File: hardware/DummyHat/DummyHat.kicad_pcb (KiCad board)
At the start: 2 copper layers, 1 part, among them U1 7404

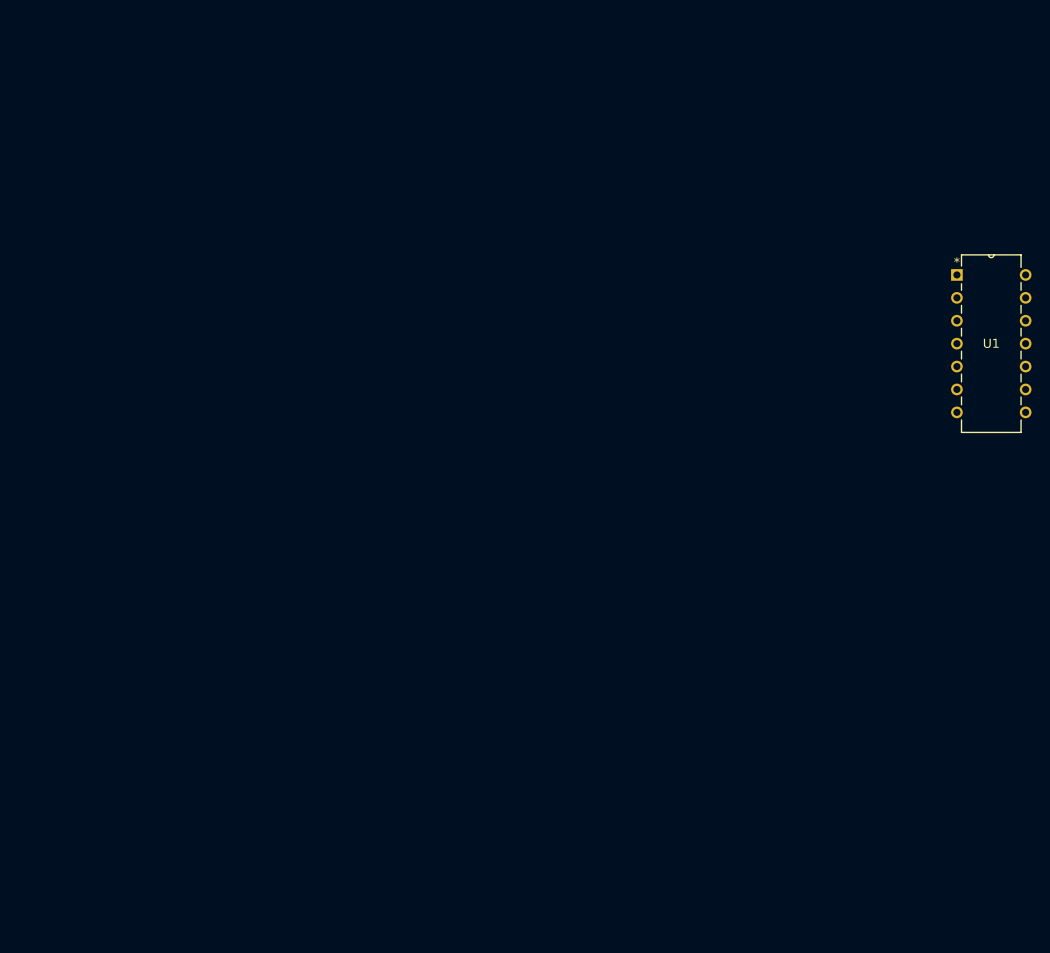
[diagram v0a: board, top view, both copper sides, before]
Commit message: Finish First Dummy Hat Design
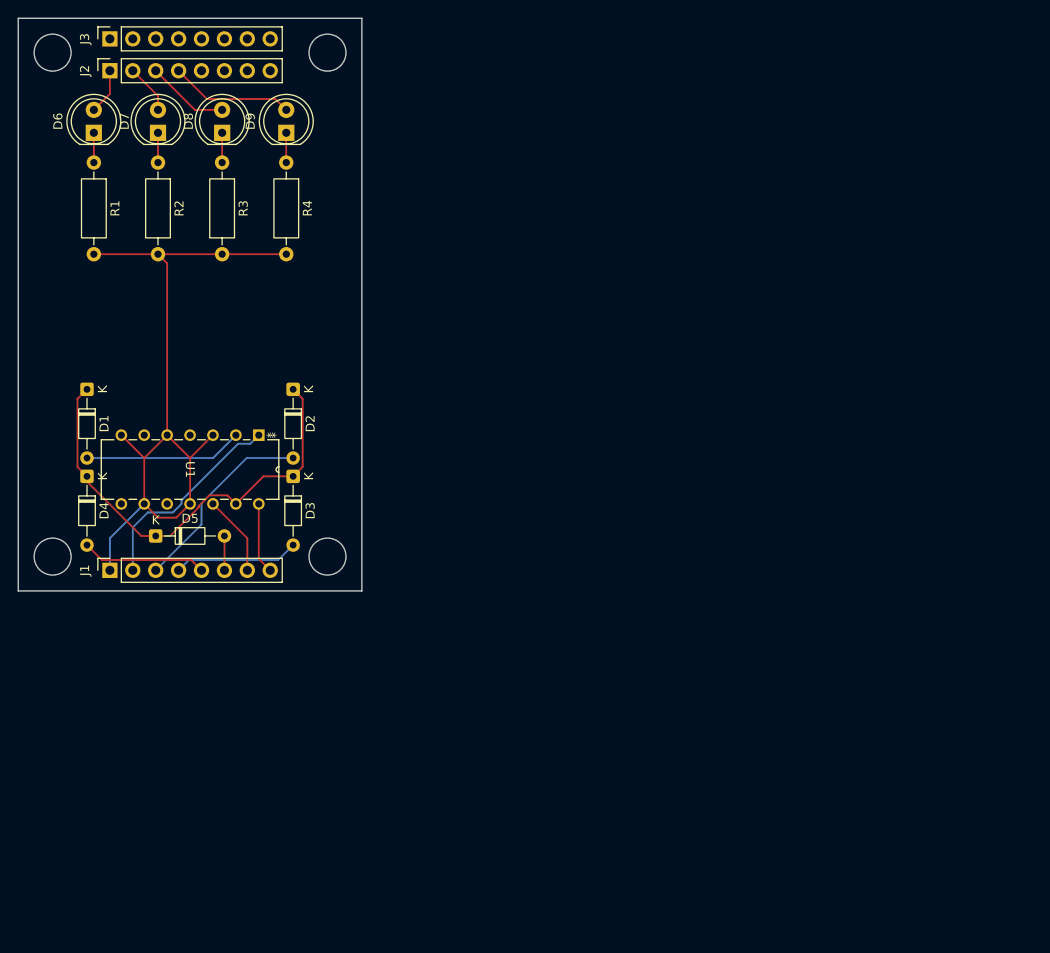
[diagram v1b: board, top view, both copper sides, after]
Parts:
- added D1: D, Diode_THT:D_DO-34_SOD68_P7.62mm_Horizontal, F.Cu at (58.4, 91.9)
- added D2: D, Diode_THT:D_DO-34_SOD68_P7.62mm_Horizontal, F.Cu at (81.3, 91.9)
- added D3: D, Diode_THT:D_DO-34_SOD68_P7.62mm_Horizontal, F.Cu at (81.3, 101.6)
- added D4: D, Diode_THT:D_DO-34_SOD68_P7.62mm_Horizontal, F.Cu at (58.4, 101.6)
- added D5: D, Diode_THT:D_DO-34_SOD68_P7.62mm_Horizontal, F.Cu at (66.0, 108.2)
- added D6: LED, LED_THT:LED_D5.0mm, F.Cu at (59.2, 63.5)
- added D7: LED, LED_THT:LED_D5.0mm, F.Cu at (66.3, 63.5)
- added D8: LED, LED_THT:LED_D5.0mm, F.Cu at (73.4, 63.5)
- added D9: LED, LED_THT:LED_D5.0mm, F.Cu at (80.5, 63.5)
- added J1: Conn_01x08_Socket, Connector_PinSocket_2.54mm:PinSocket_1x08_P2.54mm_Vertical, F.Cu at (61.0, 112.0)
- added J2: Conn_01x08_Socket, Connector_PinSocket_2.54mm:PinSocket_1x08_P2.54mm_Vertical, F.Cu at (61.0, 56.6)
- added J3: Conn_01x08_Socket, Connector_PinSocket_2.54mm:PinSocket_1x08_P2.54mm_Vertical, F.Cu at (61.0, 53.1)
- added R1: R, Resistor_THT:R_Axial_DIN0207_L6.3mm_D2.5mm_P10.16mm_Horizontal, F.Cu at (59.2, 66.8)
- added R2: R, Resistor_THT:R_Axial_DIN0207_L6.3mm_D2.5mm_P10.16mm_Horizontal, F.Cu at (66.3, 66.8)
- added R3: R, Resistor_THT:R_Axial_DIN0207_L6.3mm_D2.5mm_P10.16mm_Horizontal, F.Cu at (73.4, 66.8)
- added R4: R, Resistor_THT:R_Axial_DIN0207_L6.3mm_D2.5mm_P10.16mm_Horizontal, F.Cu at (80.5, 66.8)
- U1: value 7404 -> 74HC04
- moved U1 100.8 mm to (62.2, 104.6), turned to -90 degrees
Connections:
- U1 pad 1: unconnected-(U1-Pad1) -> I0
- U1 pad 11: unconnected-(U1-Pad11) -> GND
- U1 pad 12: unconnected-(U1-Pad12) -> RESP
- U1 pad 13: unconnected-(U1-Pad13) -> Net-(D1-K)
- U1 pad 2: unconnected-(U1-Pad2) -> Net-(D1-A)
- U1 pad 3: unconnected-(U1-Pad3) -> GND
- U1 pad 5: unconnected-(U1-Pad5) -> GND
- U1 pad 9: unconnected-(U1-Pad9) -> GND
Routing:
- net GND: track 0.00 -> 81.6 mm
- net Net-(D1-K): track 0.00 -> 50.6 mm
- net I0: track 0.00 -> 23.2 mm
- net I1: track 0.00 -> 21.8 mm
- net Net-(D1-A): track 0.00 -> 17.6 mm
- net I2: track 0.00 -> 13.9 mm
- net I3: track 0.00 -> 13.9 mm
- net D3: track 0.00 -> 13.7 mm
- net D2: track 0.00 -> 9.16 mm
- net RESP: track 0.00 -> 8.94 mm
- net +5V: track 0.00 -> 7.89 mm
- net D1: track 0.00 -> 5.50 mm
- net D0: track 0.00 -> 5.08 mm
- net I4: track 0.00 -> 3.81 mm
- net Net-(D9-K): track 0.00 -> 3.30 mm
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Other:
- board outline added: 38.1 x 63.5 mm

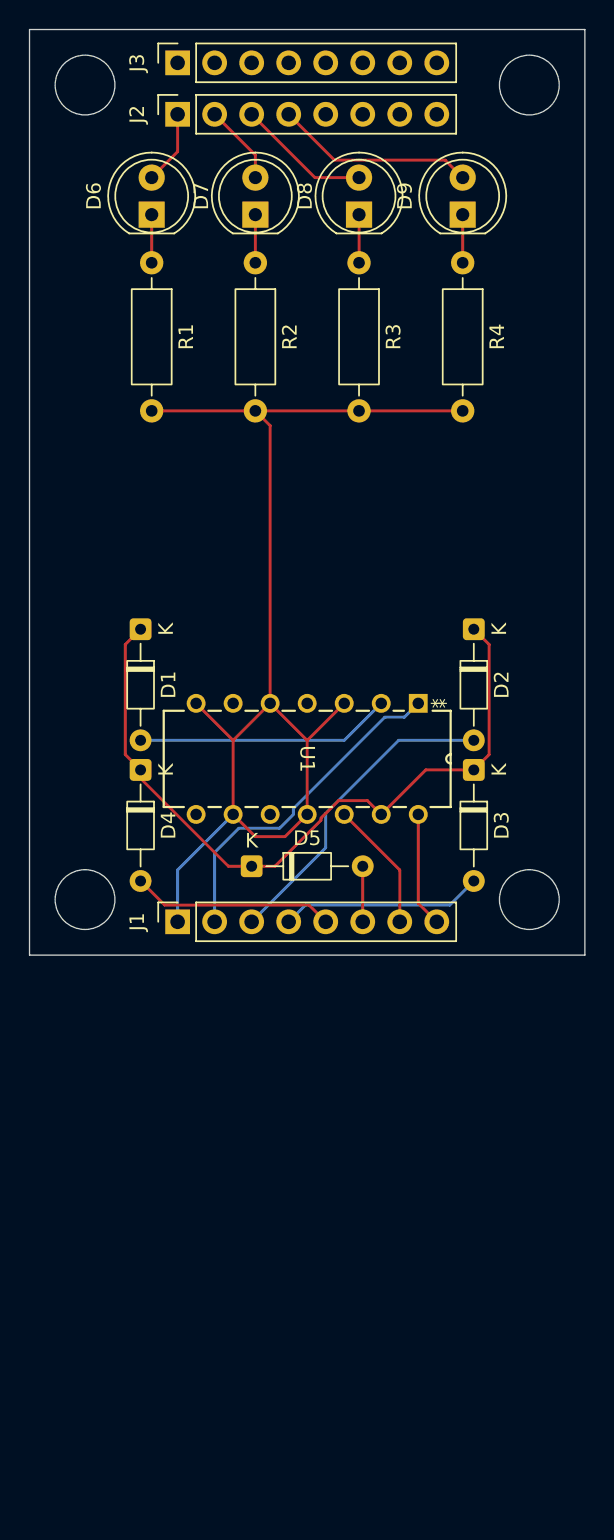
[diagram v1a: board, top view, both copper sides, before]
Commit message: Finish dev board. Limitations still apply.
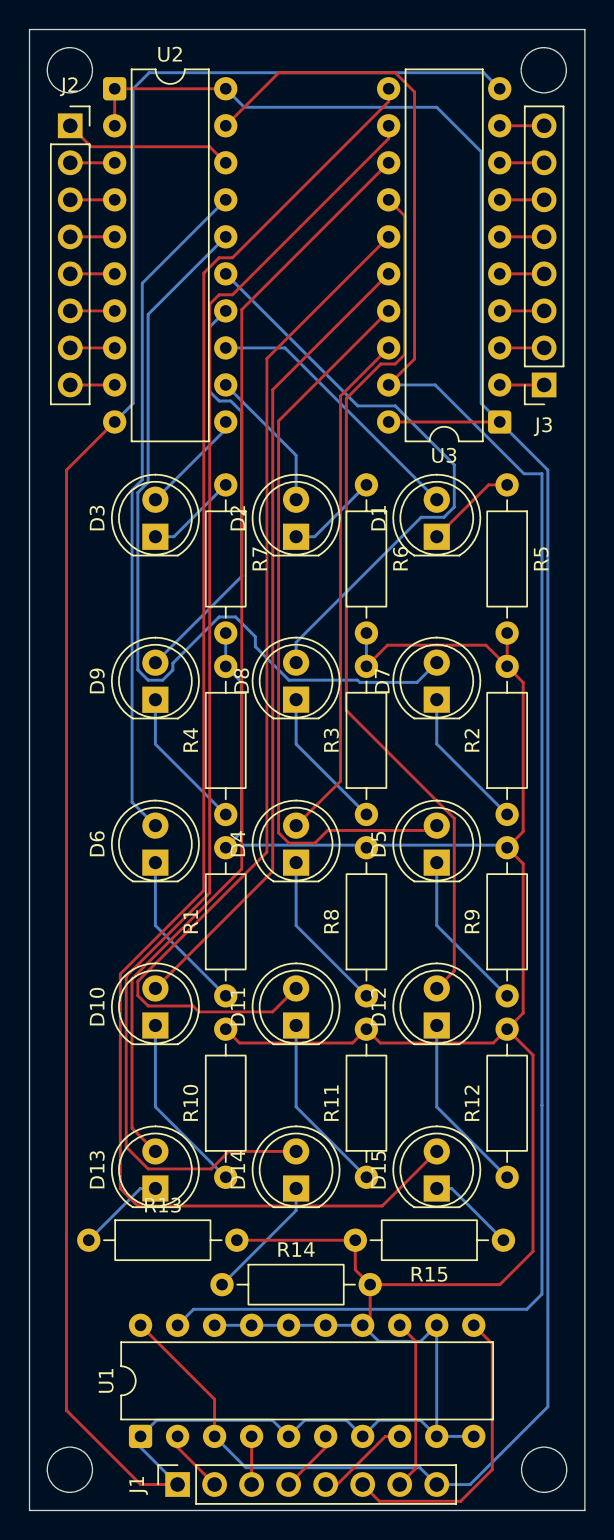
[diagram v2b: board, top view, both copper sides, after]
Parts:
- added D10: LED, LED_THT:LED_D5.0mm, F.Cu at (59.4, 119.1)
- added D11: LED, LED_THT:LED_D5.0mm, F.Cu at (69.1, 119.1)
- added D12: LED, LED_THT:LED_D5.0mm, F.Cu at (78.7, 119.1)
- added D13: LED, LED_THT:LED_D5.0mm, F.Cu at (59.4, 130.3)
- added D14: LED, LED_THT:LED_D5.0mm, F.Cu at (69.1, 130.3)
- added D15: LED, LED_THT:LED_D5.0mm, F.Cu at (78.7, 130.3)
- added R10: R, Resistor_THT:R_Axial_DIN0207_L6.3mm_D2.5mm_P10.16mm_Horizontal, F.Cu at (64.3, 129.5)
- added R11: R, Resistor_THT:R_Axial_DIN0207_L6.3mm_D2.5mm_P10.16mm_Horizontal, F.Cu at (73.9, 129.5)
- added R12: R, Resistor_THT:R_Axial_DIN0207_L6.3mm_D2.5mm_P10.16mm_Horizontal, F.Cu at (83.6, 129.5)
- added R13: R, Resistor_THT:R_Axial_DIN0207_L6.3mm_D2.5mm_P10.16mm_Horizontal, F.Cu at (54.9, 133.9)
- added R14: R, Resistor_THT:R_Axial_DIN0207_L6.3mm_D2.5mm_P10.16mm_Horizontal, F.Cu at (64.0, 136.9)
- added R15: R, Resistor_THT:R_Axial_DIN0207_L6.3mm_D2.5mm_P10.16mm_Horizontal, F.Cu at (83.3, 133.9)
- added R5: R, Resistor_THT:R_Axial_DIN0207_L6.3mm_D2.5mm_P10.16mm_Horizontal, F.Cu at (83.6, 82.0)
- added R6: R, Resistor_THT:R_Axial_DIN0207_L6.3mm_D2.5mm_P10.16mm_Horizontal, F.Cu at (73.9, 82.0)
- added R7: R, Resistor_THT:R_Axial_DIN0207_L6.3mm_D2.5mm_P10.16mm_Horizontal, F.Cu at (64.3, 82.0)
- added R8: R, Resistor_THT:R_Axial_DIN0207_L6.3mm_D2.5mm_P10.16mm_Horizontal, F.Cu at (73.9, 117.1)
- added R9: R, Resistor_THT:R_Axial_DIN0207_L6.3mm_D2.5mm_P10.16mm_Horizontal, F.Cu at (83.6, 117.1)
- added U2: 74HC245, Package_DIP:DIP-20_W7.62mm, F.Cu at (56.6, 54.9)
- added U3: 74HC245, Package_DIP:DIP-20_W7.62mm, F.Cu at (83.1, 77.7)
- D1, D2, D3, D4, D5: value D -> LED; footprint Diode_THT:D_DO-34_SOD68_P7.62mm_Horizontal -> LED_THT:LED_D5.0mm
- U1: value 74HC04 -> 74HC688; footprint 7404:N14 -> Package_DIP:DIP-20_W7.62mm
- moved R1 50.5 mm to (64.3, 117.1), turned to 90 degrees
- moved D6 44.5 mm to (59.4, 108.0)
- moved U1 42.8 mm to (58.4, 147.3), turned to 90 degrees
- moved R2 41.6 mm to (83.6, 104.6), turned to 90 degrees
- moved R4 41.2 mm to (64.3, 104.7), turned to 90 degrees
- moved D9 39.4 mm to (59.4, 96.8)
- moved J1 38.6 mm to (61.0, 150.6)
- moved R3 37.8 mm to (73.9, 104.6), turned to 90 degrees
- moved D7 35.5 mm to (78.7, 96.8)
- moved D8 33.6 mm to (69.1, 96.8)
- moved J3 33.5 mm to (86.1, 75.2), turned to 180 degrees
- moved D3 27.1 mm to (59.4, 85.6), turned to 90 degrees
- moved D1 21.3 mm to (78.7, 85.6), turned to 90 degrees
- moved D2 13.7 mm to (69.1, 85.6), turned to 90 degrees
- moved D5 12.7 mm to (78.7, 108.0), turned to 90 degrees
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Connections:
- D1 pad 2: Net-(D1-A) -> D4
- D2 pad 1: Net-(D1-K) -> Net-(D2-K)
- D2 pad 2: I1 -> D5
- D3 pad 1: Net-(D1-K) -> Net-(D3-K)
- D3 pad 2: I2 -> D6
- D4 pad 1: Net-(D1-K) -> Net-(D4-K)
- D4 pad 2: I3 -> D7
- D5 pad 1: Net-(D1-K) -> Net-(D5-K)
- D5 pad 2: I4 -> D8
- J1 pad 7: RESP -> I5
- J2 pad 1: D0 -> Net-(J2-Pin_1)
- J2 pad 2: D1 -> Net-(J2-Pin_2)
- J2 pad 3: D2 -> Net-(J2-Pin_3)
- J2 pad 4: D3 -> Net-(J2-Pin_4)
- J2 pad 5: D4 -> Net-(J2-Pin_5)
- J2 pad 6: D5 -> Net-(J2-Pin_6)
- J2 pad 7: D6 -> Net-(J2-Pin_7)
- J2 pad 8: D7 -> Net-(J2-Pin_8)
- J3 pad 1: D8 -> Net-(J3-Pin_1)
- J3 pad 2: D9 -> Net-(J3-Pin_2)
- J3 pad 3: D10 -> Net-(J3-Pin_3)
- J3 pad 4: D11 -> Net-(J3-Pin_4)
- J3 pad 5: D12 -> Net-(J3-Pin_5)
- J3 pad 6: D13 -> Net-(J3-Pin_6)
- J3 pad 7: D14 -> Net-(J3-Pin_7)
- J3 pad 8: D15 -> Net-(J3-Pin_8)
- U1 pad 1: I0 -> GND
- U1 pad 10: unconnected-(U1-Pad10) -> GND
- U1 pad 11: GND -> I4
- U1 pad 12: RESP -> GND
- U1 pad 13: Net-(D1-K) -> I5
- U1 pad 14: +5V -> GND
- U1 pad 2: Net-(D1-A) -> I0
- U1 pad 3: GND -> +5V
- U1 pad 4: unconnected-(U1-Pad4) -> I1
- U1 pad 6: unconnected-(U1-Pad6) -> I2
- U1 pad 8: unconnected-(U1-Pad8) -> I3
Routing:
- net GND: track 81.6 -> 323.3 mm
- net +5V: track 7.89 -> 161.3 mm
- net Net-(U1-P=R): track 0.00 -> 131.1 mm
- net D14: track 0.00 -> 107.4 mm
- net D13: track 0.00 -> 90.8 mm
- net D12: track 0.00 -> 75.8 mm
- net D10: track 0.00 -> 71.2 mm
- net D11: track 0.00 -> 60.4 mm
- net D9: track 0.00 -> 55.7 mm
- net D1: track 5.50 -> 57.9 mm
- net D8: track 0.00 -> 50.6 mm
- net Net-(D1-K): track 50.6 -> 6.30 mm
- net D0: track 5.08 -> 46.3 mm
- net D7: track 0.00 -> 35.4 mm
- net D2: track 9.16 -> 40.1 mm
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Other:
- board size 38.1 x 63.5 mm -> 38.1 x 101.6 mm
